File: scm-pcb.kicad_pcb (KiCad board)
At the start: 2 copper layers, 72.6 x 123.2 mm, 8 parts, among them J1 Raspberry_Pi_2_3, U2 MCP3008

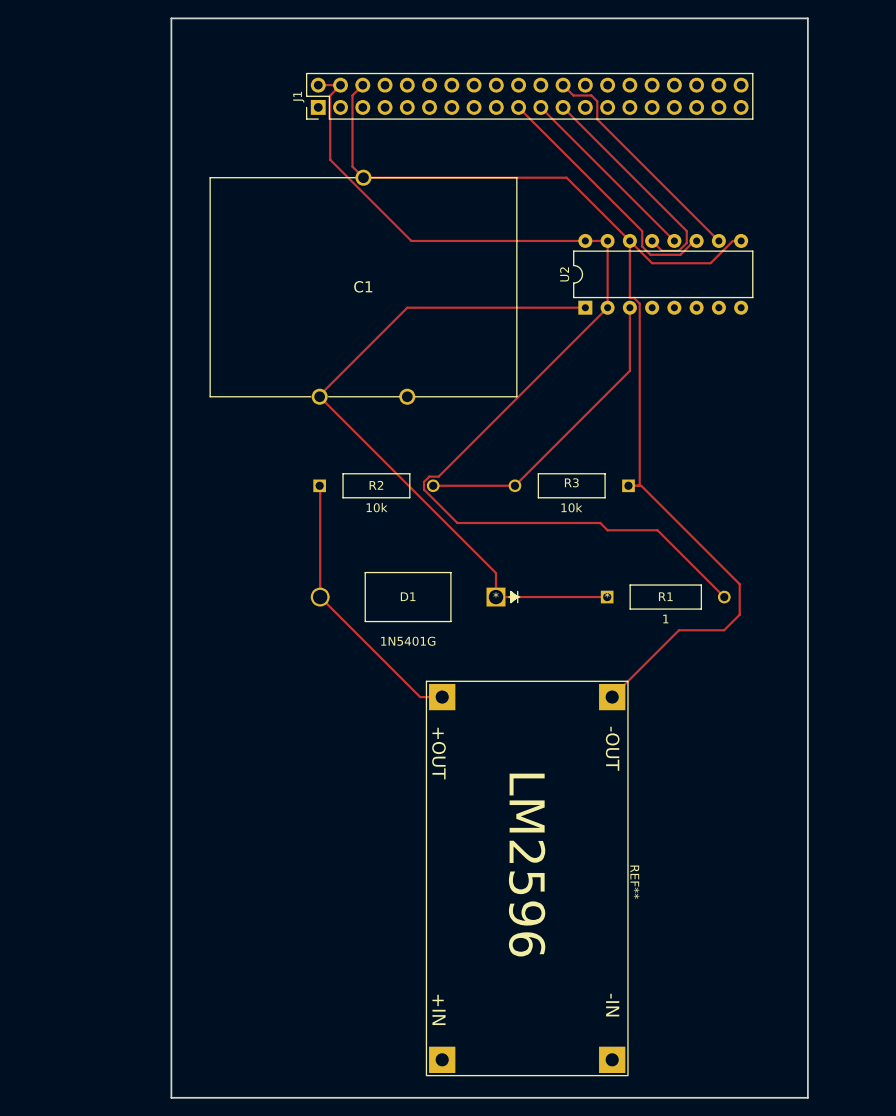
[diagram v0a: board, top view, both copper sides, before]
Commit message: Updated PCB
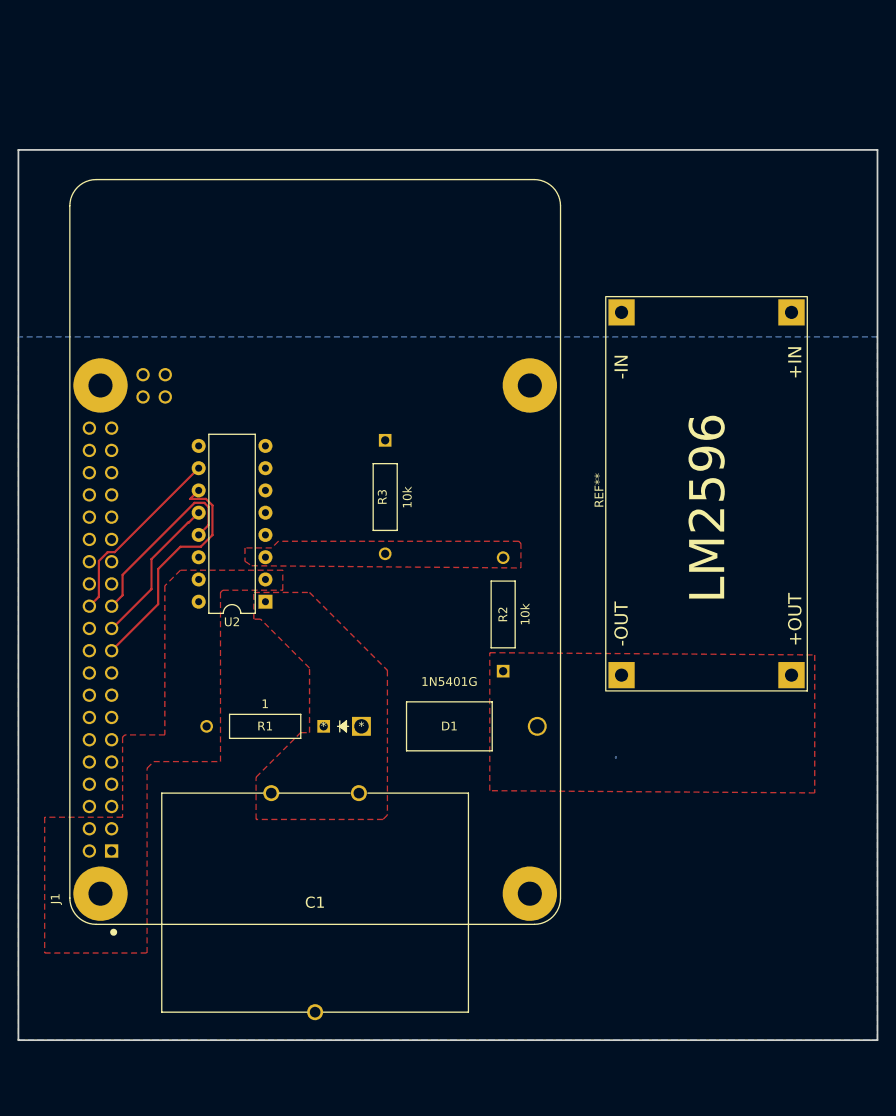
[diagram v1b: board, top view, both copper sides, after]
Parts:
- J1: footprint Connector_PinHeader_2.54mm:PinHeader_2x20_P2.54mm_Vertical -> Rpi:MODULE_RASPBERRY_PI_3_MODEL_B+
- moved J1 50.7 mm to (128.7, 86.8)
- moved U2 49.6 mm to (123.0, 92.5), turned to 180 degrees
- moved REF** 49.5 mm to (173.8, 79.8), turned to 90 degrees
- moved C1 45.5 mm to (133.7, 114.3), turned to 180 degrees
- moved R1 35.6 mm to (129.6, 106.7), turned to 180 degrees
- moved R2 29.8 mm to (150.1, 100.4), turned to 90 degrees
- moved R3 28.2 mm to (136.7, 74.1), turned to -90 degrees
- moved D1 21.3 mm to (133.9, 106.7), turned to 0 degrees
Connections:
- C1 pad 3: (no net) -> Net-(D1-K)
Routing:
- net GND: track 129.0 -> 0.00 mm
- net Net-(#FLG03-pwr): track 124.1 -> 0.00 mm
- net Net-(D1-K): track 78.7 -> 0.00 mm
- net Net-(U2-CH2): track 35.1 -> 0.00 mm
- net +6V: track 31.4 -> 0.00 mm
- net Net-(J1-~{CE0}/GPIO8): track 26.3 -> 21.4 mm
- net Net-(J1-SCLK0/GPIO11): track 26.1 -> 21.2 mm
- net Net-(J1-MISO0/GPIO9): track 21.6 -> 17.4 mm
- net Net-(J1-MOSI0/GPIO10): track 29.2 -> 26.9 mm
- added copper zone on F.Cu, net +6V
- added copper zone on B.Cu, net GND
- added copper zone on F.Cu, net Net-(#FLG03-pwr)
- added copper zone on F.Cu, net Net-(D1-K)
- added copper zone on F.Cu, net Net-(U2-CH2)
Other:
- board size 72.6 x 123.2 mm -> 98 x 101.6 mm
